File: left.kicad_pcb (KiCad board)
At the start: 2 copper layers, 152.4 x 109.7 mm, 67 parts, among them U1 74VHC4051AFT, U2 GS8051-TR, U3 ATMEGA32U4, U4 PJ-327A, Y1 Crystal

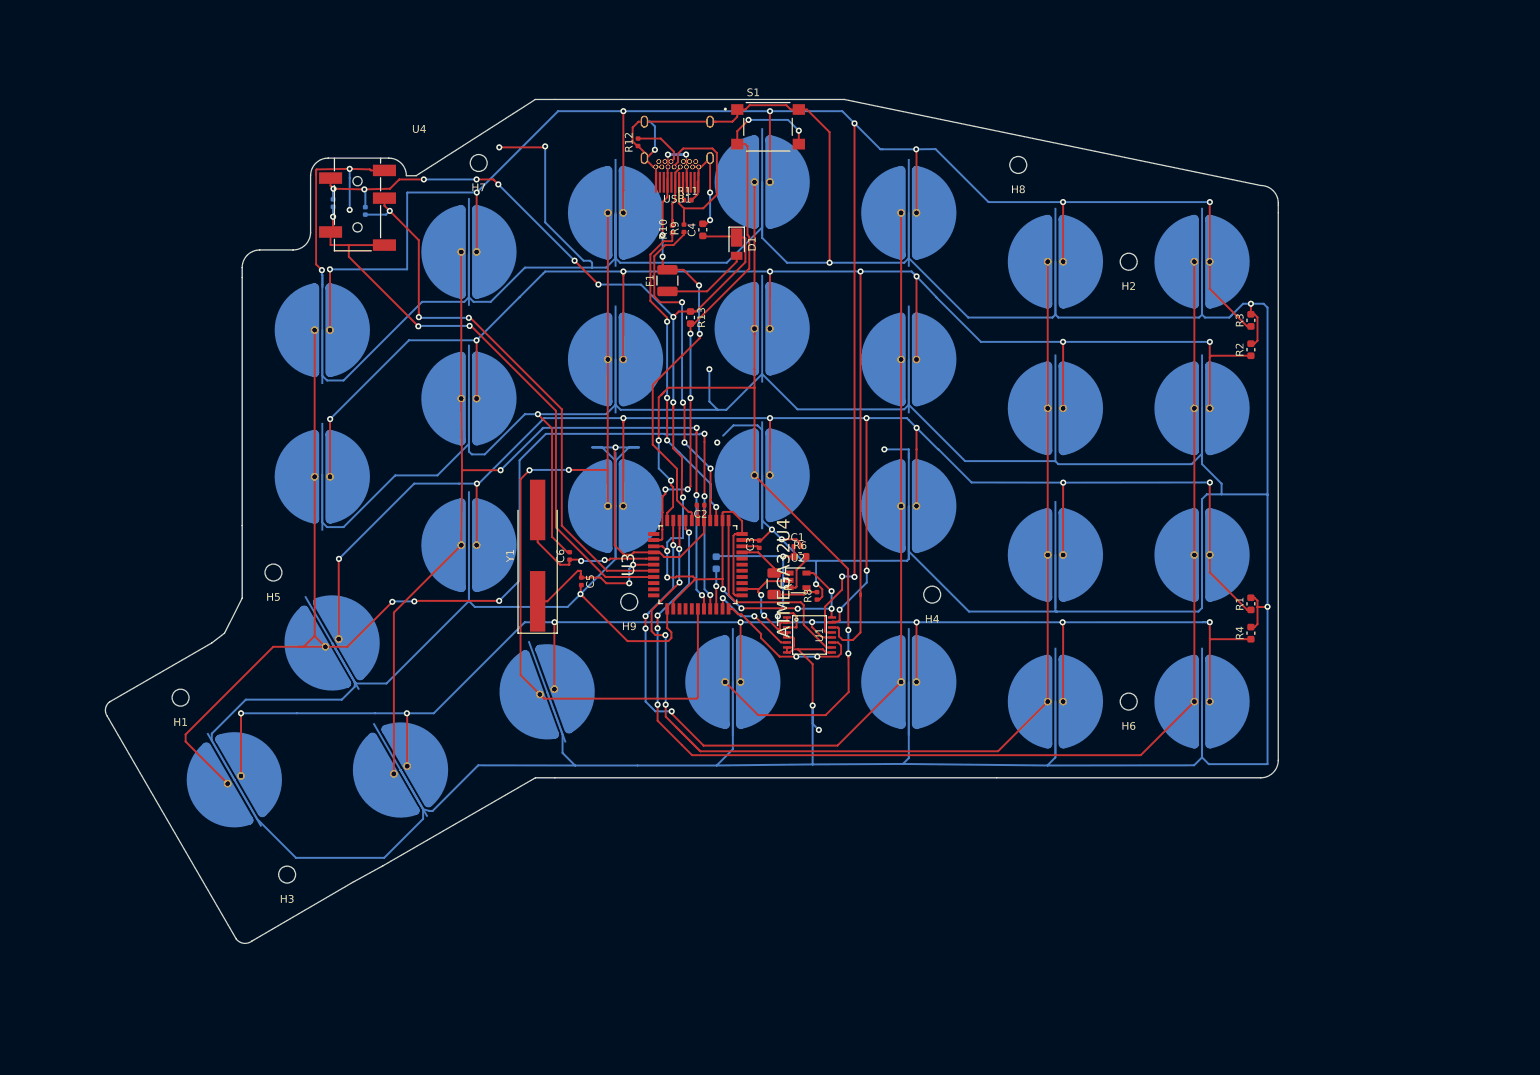
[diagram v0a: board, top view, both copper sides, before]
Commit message: fill
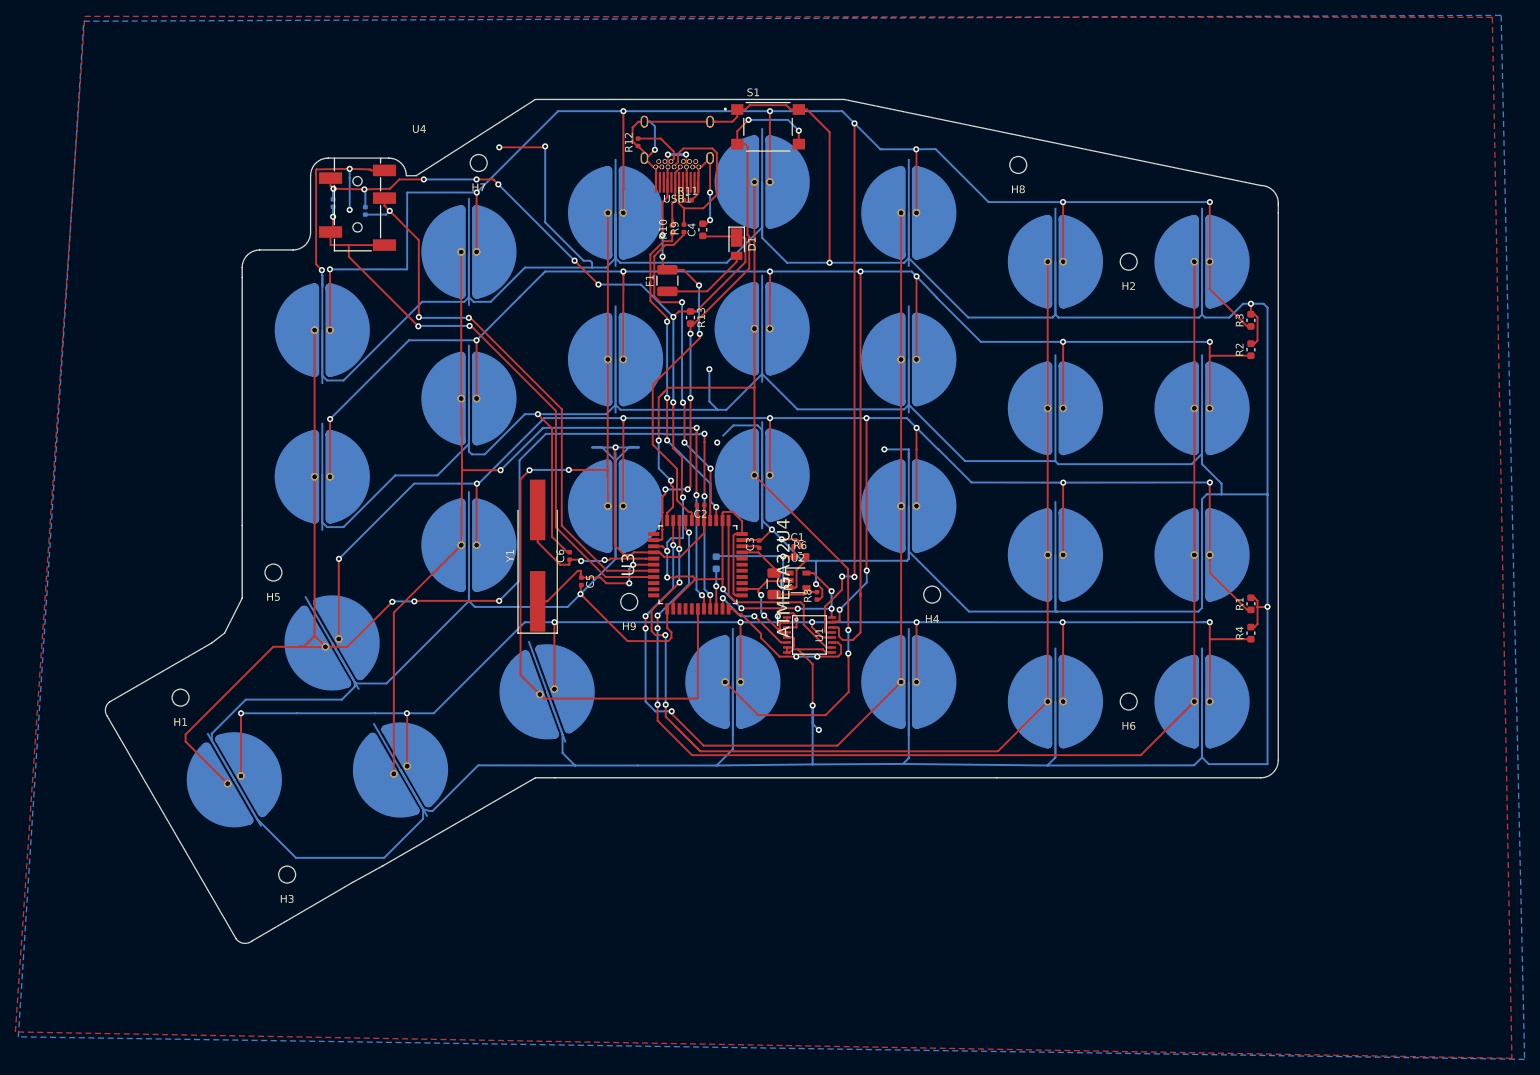
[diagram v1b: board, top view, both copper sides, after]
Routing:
- added copper zone on B.Cu, net GND
- added copper zone on F.Cu, net GND
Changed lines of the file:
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@@
+    )
+  )
+  (zone (net 1) (net_name GND) (layer F.Cu) (hatch edge 0.508)
+    (connect_pads (clearance 0.508))
+    (min_thickness 0.254)
+    (fill yes (arc_segments 32) (thermal_gap 0.508) (thermal_bridge_width 0.508))
+    (polygon
+      (pts
+        (xy 269.494 37.338) (xy 272.034 172.593) (xy 77.597 169.164) (xy 86.614 37.211)
+      )
+    )
+  )
+  (zone (net 1) (net_name GND) (layer B.Cu) (hatch edge 0.508)
+    (connect_pads (clearance 0.508))
+    (min_thickness 0.254)
+    (fill yes (arc_segments 32) (thermal_gap 0.508) (thermal_bridge_width 0.508))
+    (polygon
+      (pts
+        (xy 273.685 172.72) (xy 77.978 169.799) (xy 86.487 37.846) (xy 270.637 37.084)
+      )
     )
   )
